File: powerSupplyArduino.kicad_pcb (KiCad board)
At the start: 2 copper layers, 61 parts, among them J1 Conn_01x04, J2 Main connector, J3 Display, J4 Termo_sens, J5 ISP, J6 Encoder, U1 LM324, U2 TL494, U3 ATmega8A-AU

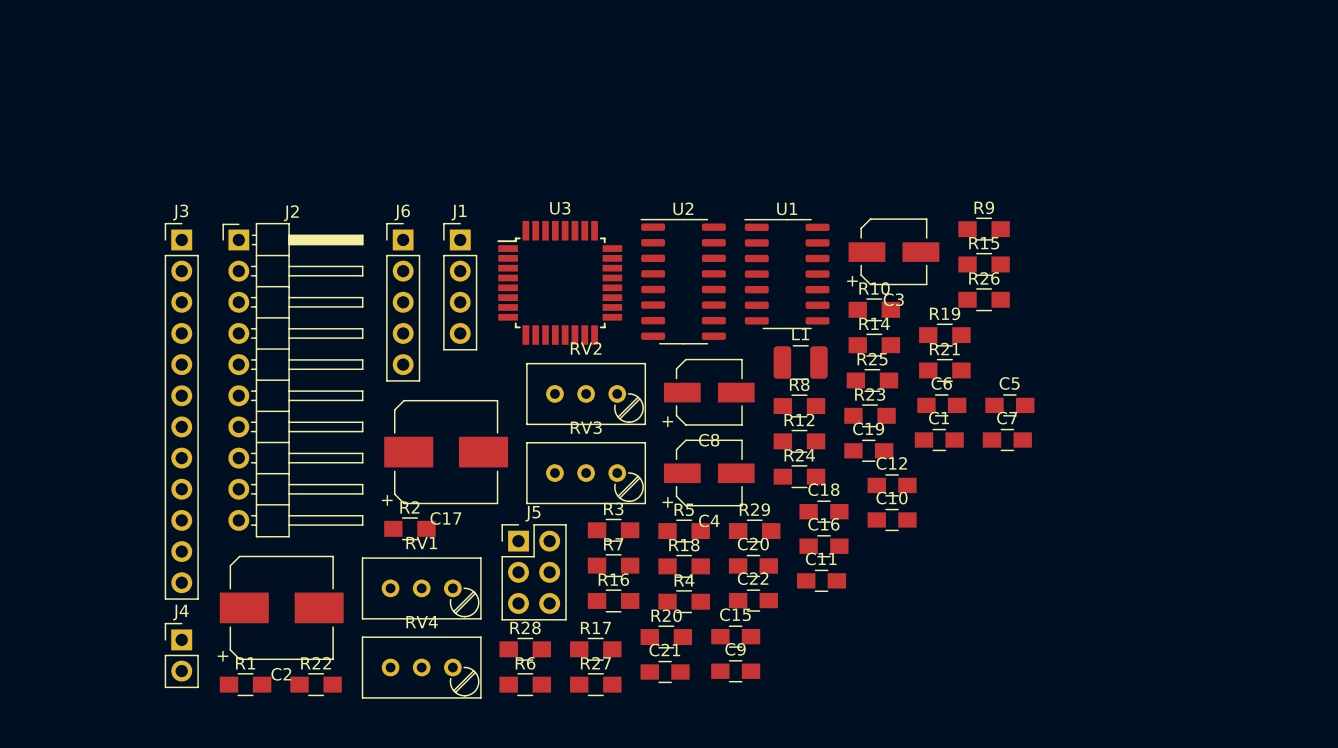
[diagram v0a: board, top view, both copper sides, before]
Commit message: first try to routing
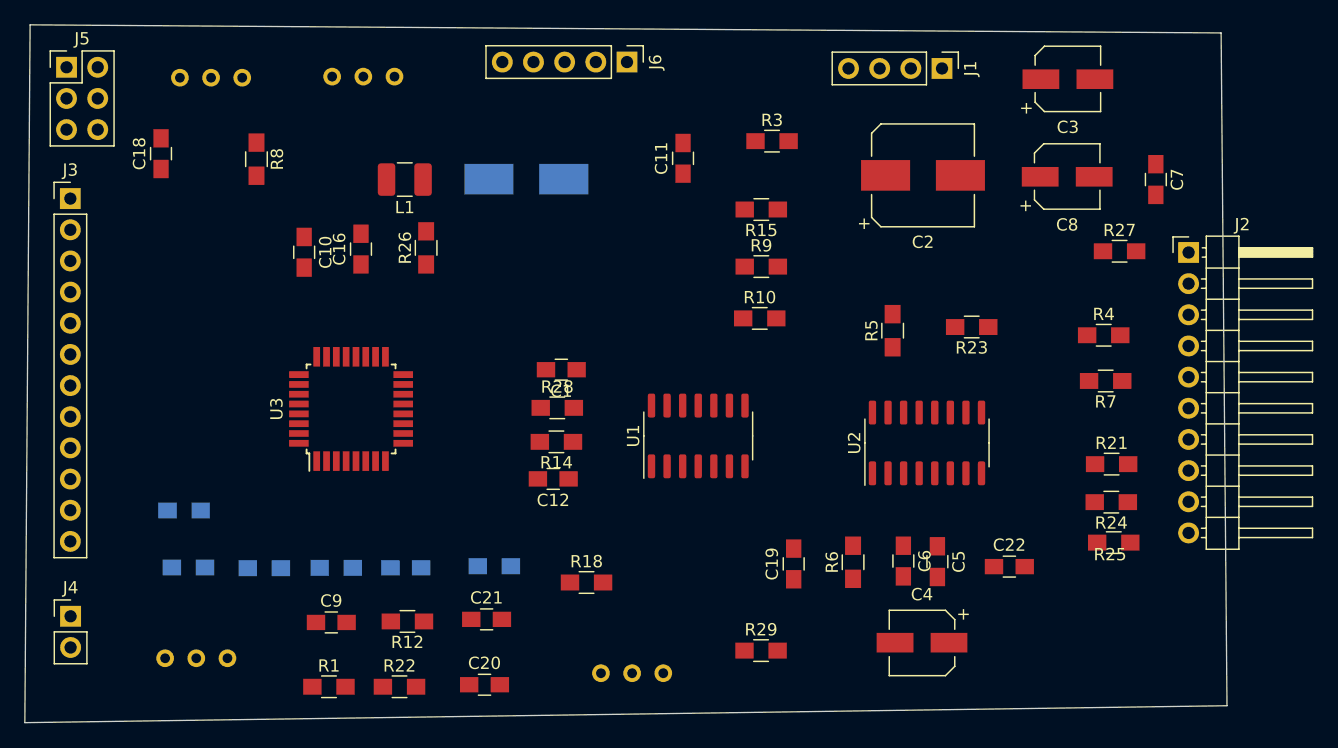
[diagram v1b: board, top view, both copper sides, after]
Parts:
- C15, C17, R16, R17, R19, R2, R20, RV1, RV2, RV3, RV4: moved to B.Cu
- moved J2 77.4 mm to (186.5, 70.0)
- moved R19 63.6 mm to (104.6, 91.0)
- moved C2 63.0 mm to (164.8, 63.7)
- moved C18 61.4 mm to (102.7, 62.0), turned to 90 degrees
- moved R27 55.4 mm to (180.9, 69.9)
- moved J5 53.4 mm to (95.0, 54.9)
- moved C10 52.7 mm to (114.4, 70.0), turned to 270 degrees
- moved R8 48.6 mm to (110.5, 62.4), turned to 270 degrees
- moved R26 45.7 mm to (124.3, 69.7), turned to 90 degrees
- moved C16 44.8 mm to (119.0, 69.8), turned to 90 degrees
- moved RV3 44.4 mm to (109.4, 55.8)
- moved R7 42.8 mm to (179.7, 80.5), turned to 180 degrees
- moved RV1 42.0 mm to (121.8, 55.7)
- moved J1 41.7 mm to (166.4, 55.0), turned to 270 degrees
- moved R4 40.5 mm to (179.6, 76.8)
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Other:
- board outline added: 98 x 56.9 mm
- net class Default: trace_width 0.25 -> 0.5; via_dia 0.8 -> 1.3; via_drill 0.4 -> 0.7
